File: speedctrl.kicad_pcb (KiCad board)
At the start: 2 copper layers, 30 parts, among them J1 Conn_01x06, J2 Conn_02x04_Odd_Even, J3 Conn_01x02, Q1 Q_NMOS_GDSD, U1 LM317L_SO8, U2 BD6231, U3 LM317L_SO8, U4 STM32F030F4Px

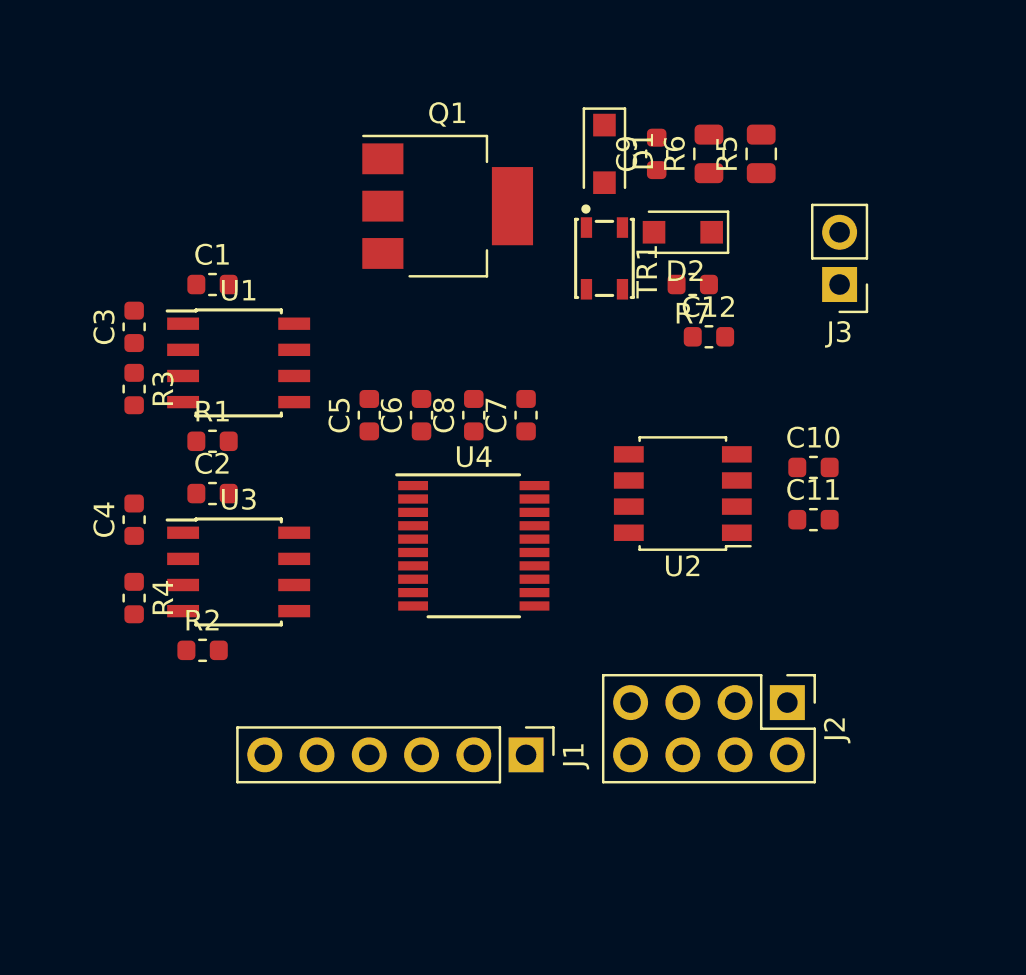
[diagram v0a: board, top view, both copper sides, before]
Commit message: Route PCB
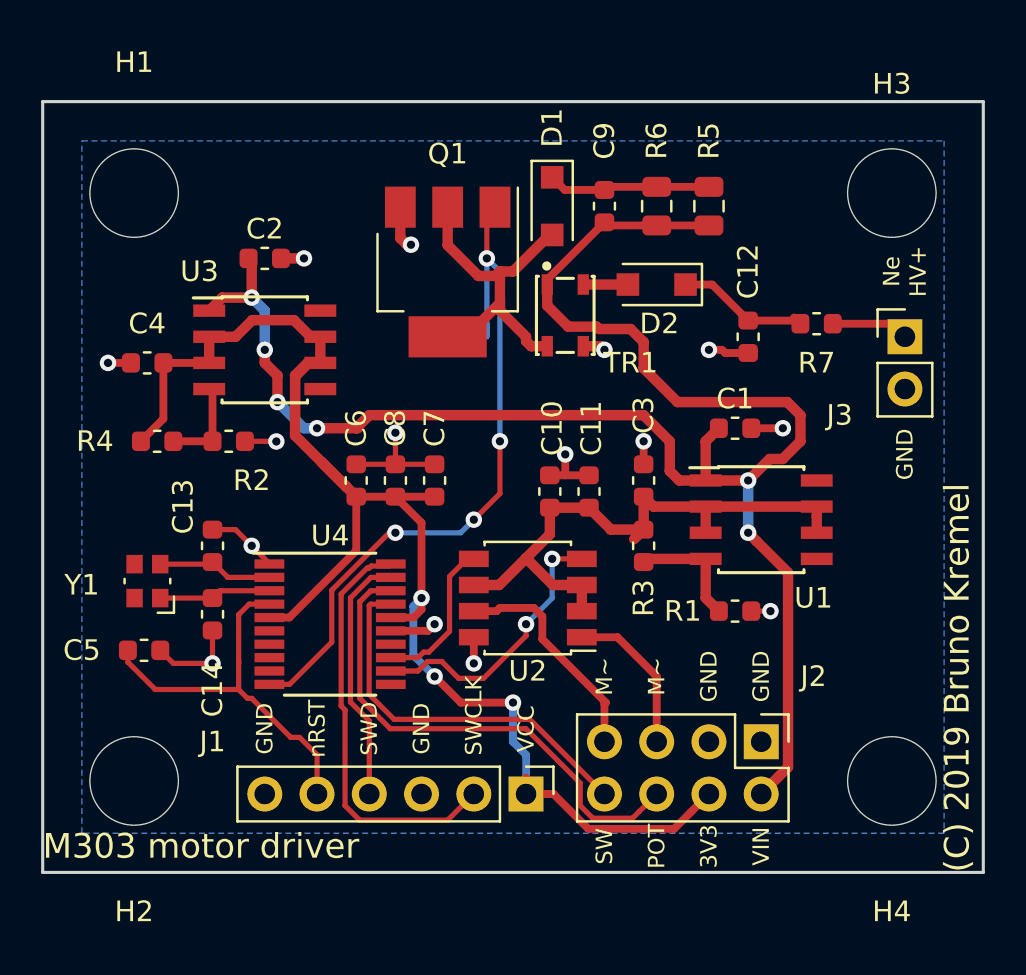
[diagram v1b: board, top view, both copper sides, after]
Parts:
- added C13: 10pF, Capacitor_SMD:C_0603_1608Metric, F.Cu at (99.1, 80.0)
- added C14: 10pF, Capacitor_SMD:C_0603_1608Metric, F.Cu at (99.1, 83.3)
- added H1: MountingHole, MountingHole:MountingHole_4.3mm_M4, F.Cu at (95.2, 62.9)
- added H2: MountingHole, MountingHole:MountingHole_4.3mm_M4, F.Cu at (95.2, 91.4)
- added H3: MountingHole, MountingHole:MountingHole_4.3mm_M4, F.Cu at (132.1, 62.9)
- added H4: MountingHole, MountingHole:MountingHole_4.3mm_M4, F.Cu at (132.1, 91.4)
- added Y1: ABM10-16MHz, Crystal:Crystal_SMD_Abracon_ABM10-4Pin_2.5x2.0mm, F.Cu at (95.9, 81.7)
- moved R1 26.7 mm to (124.5, 83.2)
- moved U1 26.5 mm to (125.7, 78.7)
- moved C1 26.3 mm to (124.5, 74.3)
- moved R3 25.9 mm to (120.0, 80.0)
- moved C3 25.9 mm to (120.0, 76.8)
- moved C5 15.8 mm to (95.7, 85.1), turned to 0 degrees
- moved C10 12.9 mm to (115.5, 77.4), turned to 90 degrees
- moved C2 11.7 mm to (101.6, 66.0)
- moved C11 11.0 mm to (117.4, 77.4), turned to 90 degrees
- moved U3 10.9 mm to (101.6, 70.5)
- moved R2 10.2 mm to (99.8, 74.9)
- moved U2 9.09 mm to (114.4, 82.5)
- moved U4 7.96 mm to (104.8, 83.8)
- moved R4 7.70 mm to (96.4, 74.9), turned to 0 degrees
- moved C4 7.65 mm to (95.9, 71.1), turned to 180 degrees
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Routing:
- net +24V: track 0.00 -> 85.4 mm, vias 0 -> 6
- net +3V3: track 0.00 -> 77.9 mm, vias 0 -> 3
- net Net-(Q1-Pad1): track 0.00 -> 35.8 mm, vias 0 -> 4
- net GND: track 0.00 -> 32.3 mm, vias 0 -> 15
- net +16V: track 0.00 -> 29.2 mm
- net /SPEED_POT_SLIDER: track 0.00 -> 24.4 mm
- net /SWCLK: track 0.00 -> 20.5 mm
- net /NRST: track 0.00 -> 19.1 mm
- net /33-45SW: track 0.00 -> 18.8 mm
- net Net-(D1-Pad2): track 0.00 -> 16.6 mm
- net Net-(U2-Pad4): track 0.00 -> 14.0 mm, vias 0 -> 2
- net /SWDIO: track 0.00 -> 12.3 mm
- net Net-(J2-Pad7): track 0.00 -> 11.0 mm
- net Net-(C9-Pad2): track 0.00 -> 7.94 mm
- net Net-(J2-Pad5): track 0.00 -> 7.60 mm
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- added copper zone on B.Cu, net GND
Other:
- board outline added: 45.7 x 37.5 mm
- rule trace_min: 0.2 -> 0.127
- rule via_min_size: 0.4 -> 0.6
- board text added: "(C) 2019 Bruno Kremel"
- board text added: "3V3"
- board text added: "GND"
- board text added: "M303 motor driver"
- board text added: "M~~"
- board text added: "Ne HV+"
- board text added: "POT"
- board text added: "SW"
- board text added: "SWCLK"
- board text added: "SWD"
- board text added: "VCC"
- board text added: "VIN"
- board text added: "nRST"
